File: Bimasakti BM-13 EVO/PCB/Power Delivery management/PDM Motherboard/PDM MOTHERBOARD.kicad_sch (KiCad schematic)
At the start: 31 parts

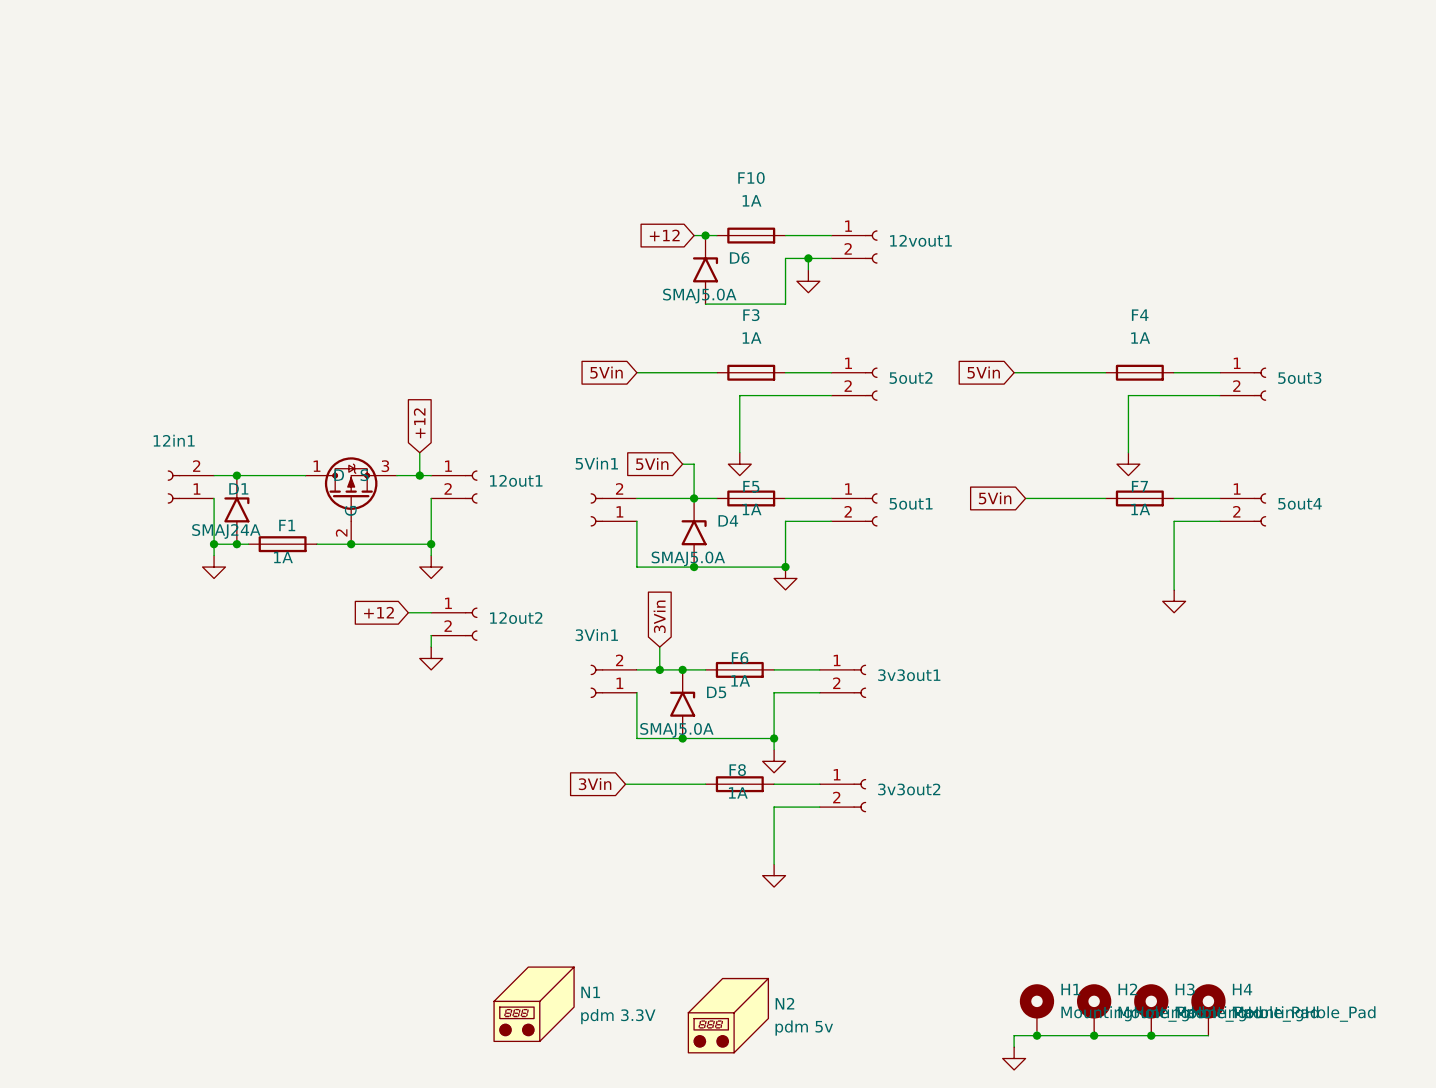
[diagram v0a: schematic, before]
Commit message: ngecilin pdm
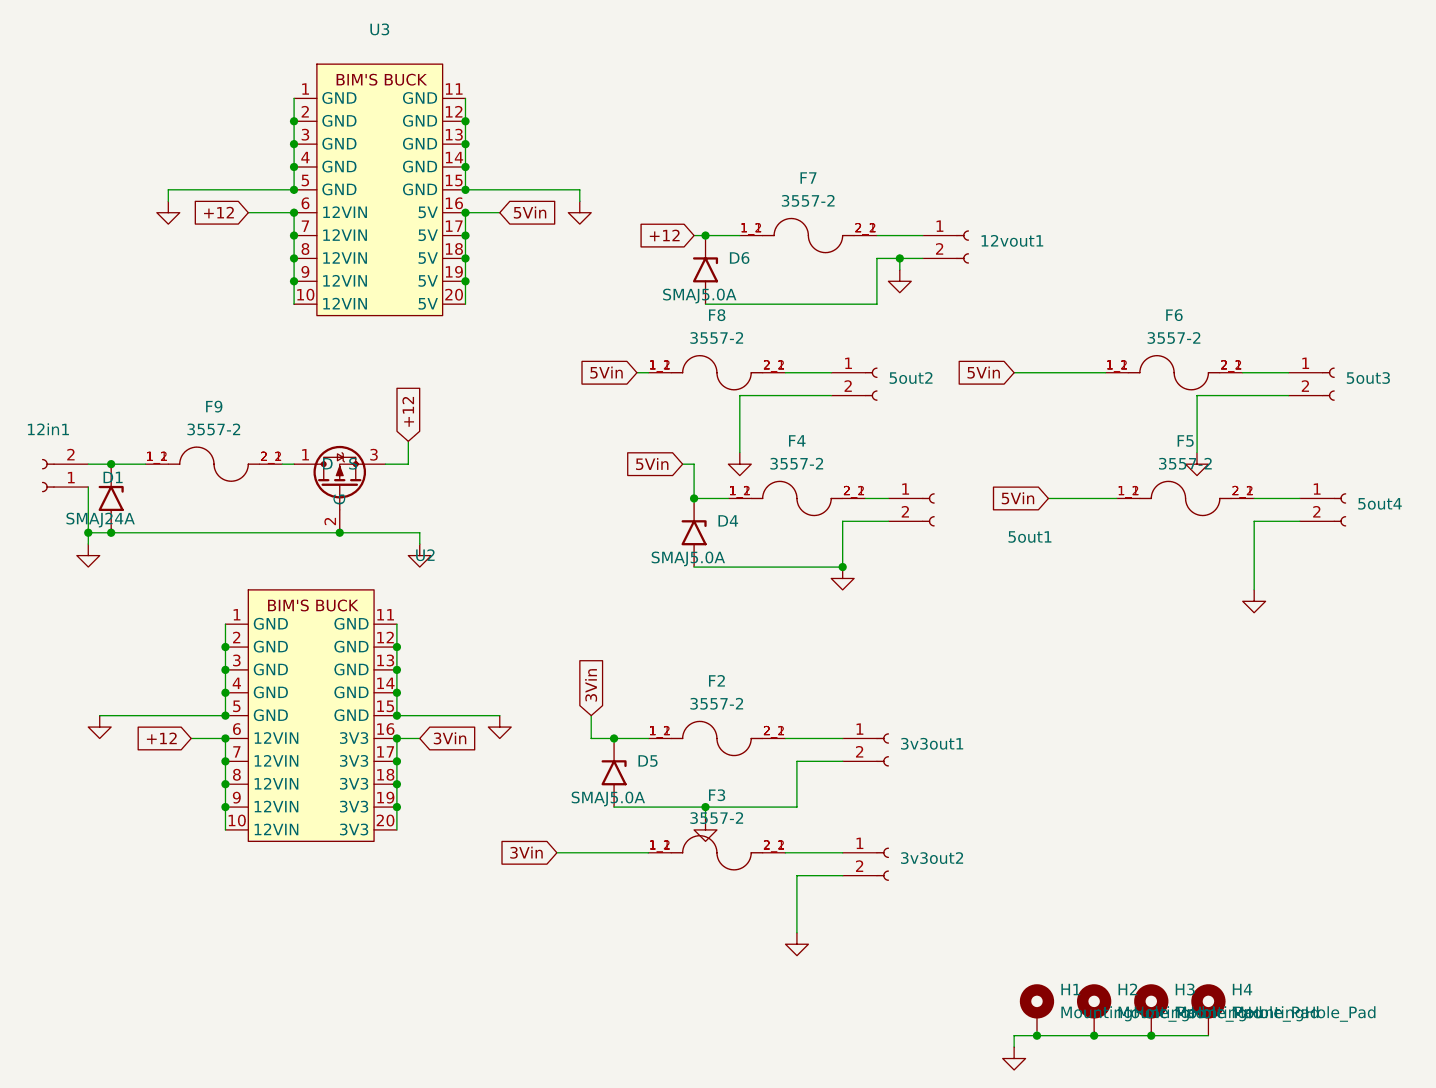
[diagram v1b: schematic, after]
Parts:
- removed 12out1, 12out2, 3Vin1, 5Vin1: ~, Connector_JST:JST_EH_B2B-EH-A_1x02_P2.50mm_Vertical, symbol Connector:Conn_01x02_Socket
- removed F1, F10, F3, F4, F5, F6, F7, F8: 1A, Fuse:Fuseholder_Cylinder-5x20mm_Schurter_0031_8201_Horizontal_Open, symbol Device:Fuse
- removed N1: pdm 3.3V, Symbol:OSHW-Symbol_6.7x6mm_SilkScreen, symbol Mechanical:Housing
- removed N2: pdm 5v, Symbol:OSHW-Symbol_6.7x6mm_SilkScreen, symbol Mechanical:Housing
- added F2, F3, F4, F5, F6, F7, F8, F9: 3557-2, 0_FUSE:0_FUSE_3557-2, symbol 0_fuse_3557-2:3557-2
- added U2: ~, BIMS_BUCK:BIMS_BUCK, symbol 0_BUCK:BIMS_BUCK_3V3
- added U3: ~, BIMS_BUCK:BIMS_BUCK, symbol 0_BUCK:BIMS_BUCK_5V
- 12in1: footprint Connector_JST:JST_EH_B2B-EH-A_1x02_P2.50mm_Vertical -> TerminalBlock_TE-Connectivity:TerminalBlock_TE_282834-2_1x02_P2.54mm_Horizontal
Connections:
- net +12: now also F7.1_1, F7.1_2, U2.10 (12VIN), U2.6 (12VIN), U2.7 (12VIN), U2.8 (12VIN), U2.9 (12VIN), U3.10 (12VIN), U3.6 (12VIN), U3.7 (12VIN), U3.8 (12VIN), U3.9 (12VIN)
- net 3Vin: now also F2.1_1, F2.1_2, F3.1_1, F3.1_2, U2.16 (3V3), U2.17 (3V3), U2.18 (3V3), U2.19 (3V3), U2.20 (3V3)
- net 5Vin: now also F4.1_1, F4.1_2, F5.1_1, F5.1_2, F6.1_1, F6.1_2, F8.1_1, F8.1_2, U3.16 (5V), U3.17 (5V), U3.18 (5V), U3.19 (5V), U3.20 (5V)
- net GND: now also U2.1 (GND), U2.11 (GND), U2.12 (GND), U2.13 (GND), U2.14 (GND), U2.15 (GND), U2.2 (GND), U2.3 (GND), U2.4 (GND), U2.5 (GND), U3.1 (GND), U3.11 (GND), U3.12 (GND), U3.13 (GND), U3.14 (GND), U3.15 (GND), U3.2 (GND), U3.3 (GND), U3.4 (GND), U3.5 (GND)
- net at 3v3out2.1 (Pin_1): now also F3.2_1, F3.2_2
- net at 12in1.2 (Pin_2), D1.1 (A1): now also F9.1_1, F9.1_2; no longer U1.1 (D)
- net at 12vout1.1 (Pin_1): now also F7.2_1, F7.2_2
- net at 5out3.1 (Pin_1): now also F6.2_1, F6.2_2
- net at 5out2.1 (Pin_1): now also F8.2_1, F8.2_2
- net at 5out1.1 (Pin_1): now also F4.2_1, F4.2_2
- net at 5out4.1 (Pin_1): now also F5.2_1, F5.2_2
- net at 3v3out1.1 (Pin_1): now also F2.2_1, F2.2_2
- new net: F9.2_1, F9.2_2, U1.1 (D)
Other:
- moved on the sheet: 12in1, 12vout1, 3v3out1, 3v3out2, 5out1, 5out3, 5out4, D1, D5
